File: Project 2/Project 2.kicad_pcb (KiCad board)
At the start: 2 copper layers, 114.6 x 108.5 mm, 63 parts, among them J1 USB_B, J2 Jack-DC, J3 BLDC_Output, J4 Servo_1, J5 Bluetooth, J6 LCD, J7 Servo_2, Q1 IRF540N, Q2 IRF540N, Q3 IRF540N, Q4 IRF540N, Q5 IRF540N, Q6 IRF540N, SW1 Reset_Button, U1 ATmega2560-16A, U2 L7805, U3 IR2104, U4 IR2104, U5 IR2104, U6 mystery_uart_thing, Y1 Crystal

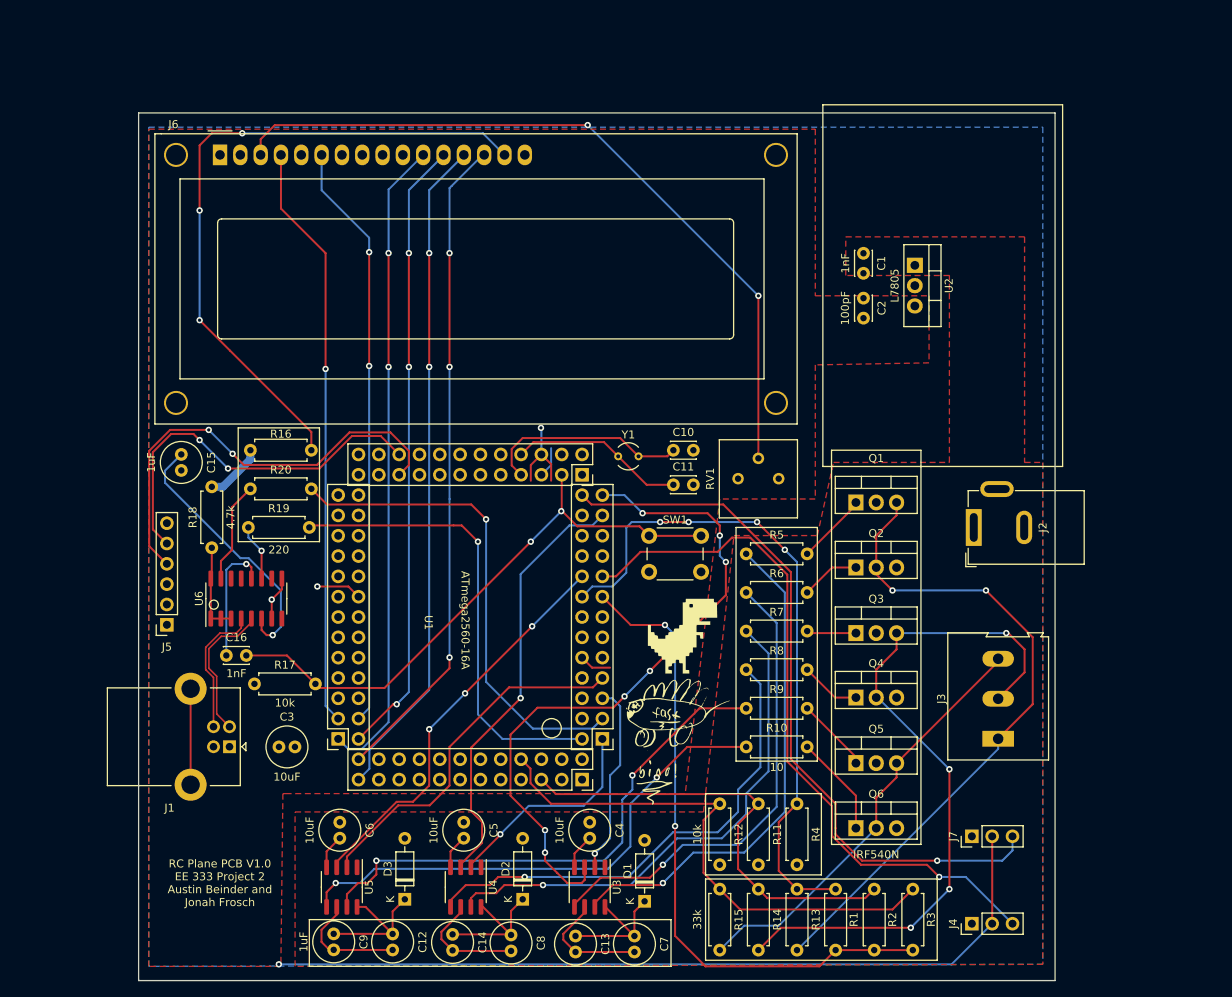
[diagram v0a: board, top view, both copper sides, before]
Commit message: added current pcb
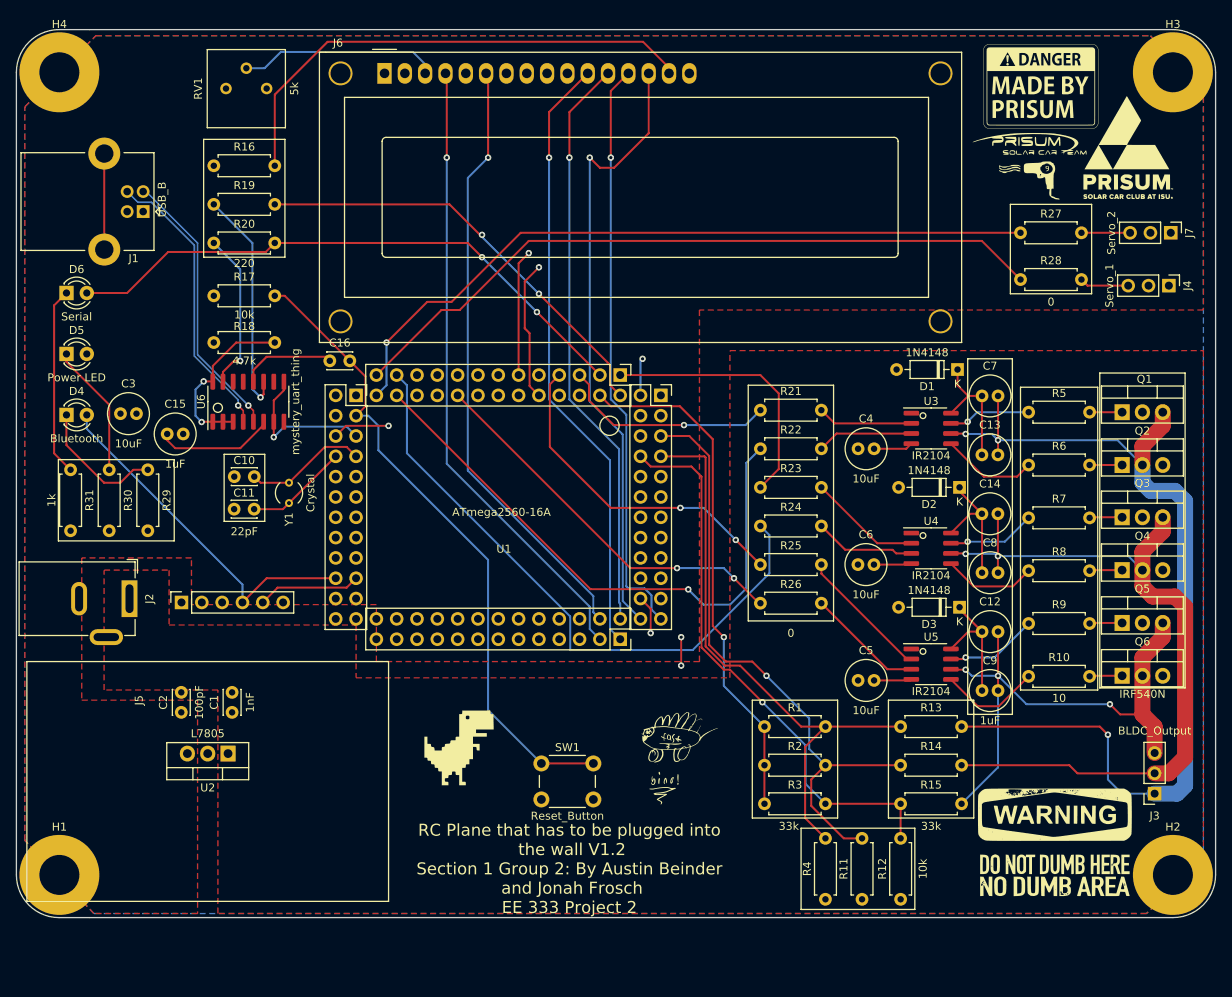
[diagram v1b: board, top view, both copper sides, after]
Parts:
- removed the G*** at (150.6, 118.9)
- removed the G*** at (151.4, 105.4)
- added D4: Bluetooth, LED_THT:LED_D3.0mm, F.Cu at (74.3, 77.9)
- added D5: Power LED, LED_THT:LED_D3.0mm, F.Cu at (74.3, 70.3)
- added D6: Serial, LED_THT:LED_D3.0mm, F.Cu at (74.3, 62.6)
- added G***: LOGO, LOGO, F.Cu at (123.4, 119.4)
- added G***: LOGO, LOGO, F.Cu at (197.9, 131.3)
- added G***: LOGO, LOGO, F.Cu at (150.9, 120.9)
- added G***: LOGO, LOGO, F.Cu at (207.0, 44.5)
- added G***: LOGO, LOGO, F.Cu at (196.1, 36.8)
- added G***: LOGO, LOGO, F.Cu at (194.8, 46.7)
- added H1: MountingHole, MountingHole:MountingHole_5mm_Pad, F.Cu at (73.4, 135.4)
- added H2: MountingHole, MountingHole:MountingHole_5mm_Pad, F.Cu at (212.6, 135.4)
- added H3: MountingHole, MountingHole:MountingHole_5mm_Pad, F.Cu at (212.6, 35.1)
- added H4: MountingHole, MountingHole:MountingHole_5mm_Pad, F.Cu at (73.4, 35.1)
- added R21: 0, Resistor_THT:R_Axial_DIN0207_L6.3mm_D2.5mm_P7.62mm_Horizontal, F.Cu at (161.0, 77.3)
- added R22: 0, Resistor_THT:R_Axial_DIN0207_L6.3mm_D2.5mm_P7.62mm_Horizontal, F.Cu at (161.0, 82.1)
- added R23: 0, Resistor_THT:R_Axial_DIN0207_L6.3mm_D2.5mm_P7.62mm_Horizontal, F.Cu at (161.0, 86.9)
- added R24: 0, Resistor_THT:R_Axial_DIN0207_L6.3mm_D2.5mm_P7.62mm_Horizontal, F.Cu at (161.0, 91.8)
- added R25: 0, Resistor_THT:R_Axial_DIN0207_L6.3mm_D2.5mm_P7.62mm_Horizontal, F.Cu at (161.0, 96.6)
- added R26: 0, Resistor_THT:R_Axial_DIN0207_L6.3mm_D2.5mm_P7.62mm_Horizontal, F.Cu at (161.0, 101.4)
- added R27: 0, Resistor_THT:R_Axial_DIN0207_L6.3mm_D2.5mm_P7.62mm_Horizontal, F.Cu at (193.5, 55.1)
- added R28: 0, Resistor_THT:R_Axial_DIN0207_L6.3mm_D2.5mm_P7.62mm_Horizontal, F.Cu at (193.5, 61.0)
- added R29: 1k, Resistor_THT:R_Axial_DIN0207_L6.3mm_D2.5mm_P7.62mm_Horizontal, F.Cu at (84.5, 84.7)
- added R30: 1k, Resistor_THT:R_Axial_DIN0207_L6.3mm_D2.5mm_P7.62mm_Horizontal, F.Cu at (79.6, 84.7)
- added R31: 1k, Resistor_THT:R_Axial_DIN0207_L6.3mm_D2.5mm_P7.62mm_Horizontal, F.Cu at (74.8, 84.7)
- J3: footprint TerminalBlock:TerminalBlock_Altech_AK300-3_P5.00mm -> Connector_PinSocket_2.54mm:PinSocket_1x03_P2.54mm_Vertical
- moved J2 105.9 mm to (82.2, 100.9), turned to -90 degrees
- moved U2 105.3 mm to (94.5, 120.2), turned to 180 degrees
- moved C2 98.5 mm to (88.6, 115.1)
- moved C1 97.6 mm to (95.0, 115.1), turned to 90 degrees
- moved C9 86.6 mm to (188.7, 112.3), turned to 0 degrees
- moved C14 84.5 mm to (188.7, 90.2), turned to 0 degrees
- moved J4 83.5 mm to (212.1, 61.7), turned to -90 degrees
- moved C12 82.8 mm to (188.7, 105.0), turned to 0 degrees
- moved RV1 80.5 mm to (99.3, 37.1)
- moved C7 80.3 mm to (188.7, 75.5), turned to 0 degrees
- moved J7 79.4 mm to (212.3, 55.1), turned to -90 degrees
- moved U5 78.8 mm to (182.4, 109.0), turned to 0 degrees
- moved C13 78.7 mm to (188.7, 82.9), turned to 0 degrees
- moved D3 78.4 mm to (185.9, 101.9), turned to 180 degrees
- moved D1 77.1 mm to (185.7, 72.2), turned to 180 degrees
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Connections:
- J3 pad 1: Net-(J3-Pad1) -> Net-(C13-Pad2)
- J3 pad 2: Net-(J3-Pad2) -> Net-(C14-Pad2)
- J3 pad 3: Net-(J3-Pad3) -> Net-(C12-Pad2)
- J4 pad 3: 8 -> Net-(J4-Pad3)
- J7 pad 3: 13 -> Net-(J7-Pad3)
- Q1 pad 3: Net-(J3-Pad1) -> Net-(C13-Pad2)
- Q2 pad 2: Net-(J3-Pad1) -> Net-(C13-Pad2)
- Q3 pad 3: Net-(J3-Pad2) -> Net-(C14-Pad2)
- Q4 pad 2: Net-(J3-Pad2) -> Net-(C14-Pad2)
- Q5 pad 3: Net-(J3-Pad3) -> Net-(C12-Pad2)
- Q6 pad 2: Net-(J3-Pad3) -> Net-(C12-Pad2)
- R1 pad 1: 6 -> pin 4
- R1 pad 2: 7 -> A4
- R13 pad 1: 7 -> A4
- R13 pad 2: Net-(J3-Pad1) -> Net-(C13-Pad2)
- R14 pad 2: Net-(J3-Pad2) -> Net-(C14-Pad2)
- R15 pad 2: Net-(J3-Pad3) -> Net-(C12-Pad2)
- R2 pad 1: 6 -> pin 4
- R3 pad 1: 6 -> pin 4
- R4 pad 1: 7 -> A4
- U1 pad 15: 6 -> unconnected-(U1-Pad15)
- U1 pad 16: 7 -> unconnected-(U1-Pad16)
- U1 pad 17: 8 -> unconnected-(U1-Pad17)
- U1 pad 24: unconnected-(U1-Pad24) -> 11
- U1 pad 4: unconnected-(U1-Pad4) -> pin 4
- U1 pad 45: Rx1 -> Tx1
- U1 pad 46: Tx1 -> Rx1
- U1 pad 93: unconnected-(U1-Pad93) -> A4
- U3 pad 2: 5 -> Net-(R21-Pad2)
- U3 pad 3: 12 -> Net-(R22-Pad2)
- U4 pad 2: 4 -> Net-(R23-Pad2)
- U4 pad 3: 10 -> Net-(R24-Pad2)
- U5 pad 2: 3 -> Net-(R25-Pad2)
- U5 pad 3: 9 -> Net-(R26-Pad2)
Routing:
- net Net-(C13-Pad2): track 14.7 -> 119.8 mm, vias 0 -> 3
- net +5V: track 124.6 -> 34.3 mm, vias 2 -> 4
- net 8: track 89.1 -> 0.00 mm, vias 1 -> 0
- net Net-(J3-Pad2): track 88.4 -> 0.00 mm, vias 4 -> 0
- net Net-(J3-Pad1): track 84.2 -> 0.00 mm, vias 2 -> 0
- net 7: track 83.7 -> 0.00 mm, vias 4 -> 0
- net Net-(C14-Pad2): track 14.4 -> 96.3 mm, vias 0 -> 2
- net 6: track 80.8 -> 0.00 mm, vias 2 -> 0
- net A4: track 0.00 -> 73.9 mm
- net 11: track 0.00 -> 73.6 mm, vias 0 -> 1
- net Net-(J6-Pad3): track 94.1 -> 25.0 mm, vias 2 -> 0
- net pin 4: track 0.00 -> 64.6 mm, vias 0 -> 1
- net Net-(R9-Pad1): track 66.3 -> 11.6 mm, vias 2 -> 1
- net Net-(R7-Pad1): track 65.0 -> 11.0 mm
- net Net-(J3-Pad3): track 53.4 -> 0.00 mm
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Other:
- board size 114.6 x 108.5 mm -> 149.9 x 111 mm
- board text added: "RC Plane that has to be plugged into the wall V1.2 Section 1 Group 2: By Austin Beinder and Jonah Frosch EE 333 Project 2"
- board text removed: "According to all known laws of aviation, there is no way that a bee should be able to fly. Its wings are too small to get its fat little body off the ground. The bee, of course, flies anyway. Because bees don't care what humans think is impossible.{dblquote} SEQ. 75 - {dblquote}INTRO TO BARRY{dblquote} INT. BENSON HOUSE - DAY ANGLE ON: Sneakers on the ground. Camera PANS UP to reveal BARRY BENSON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"
- board text removed: "RC Plane PCB V1.0 EE 333 Project 2 Austin Beinder and Jonah Frosch"
